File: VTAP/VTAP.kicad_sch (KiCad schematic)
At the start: 40 parts, among them J1 MX 52901-0274

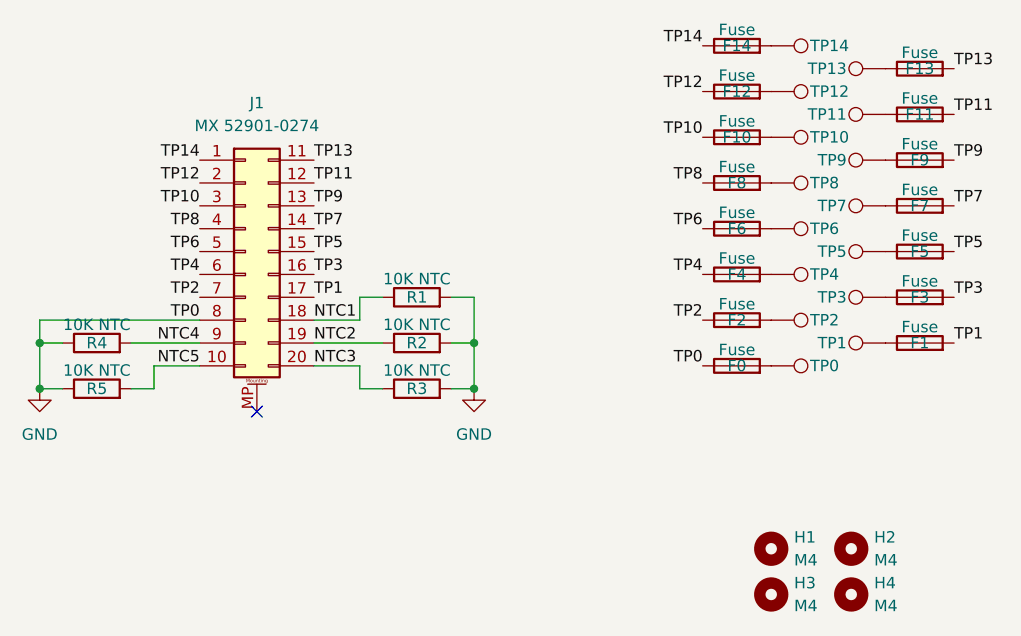
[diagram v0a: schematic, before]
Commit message: VTAP update
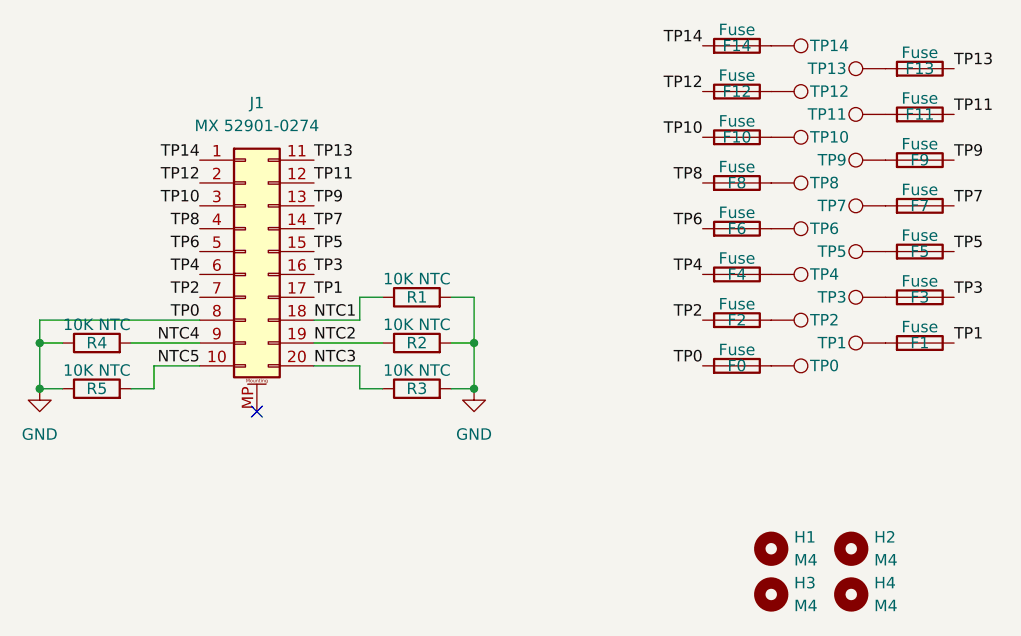
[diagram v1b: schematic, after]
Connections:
- net GND: now also F0.2; no longer F0.1
- net TP1: now also F1.1; no longer F1.2
- net TP10: now also F10.2; no longer F10.1
- net TP11: now also F11.1; no longer F11.2
- net TP12: now also F12.2; no longer F12.1
- net TP13: now also F13.1; no longer F13.2
- net TP14: now also F14.2; no longer F14.1
- net TP2: now also F2.2; no longer F2.1
- net TP3: now also F3.1; no longer F3.2
- net TP4: now also F4.2; no longer F4.1
- net TP5: now also F5.1; no longer F5.2
- net TP6: now also F6.2; no longer F6.1
- net TP7: now also F7.1; no longer F7.2
- net TP8: now also F8.2; no longer F8.1
- net TP9: now also F9.1; no longer F9.2
- net at TP12.1: now also F12.1; no longer F12.2
- net at TP1.1: now also F1.2; no longer F1.1
- net at TP13.1: now also F13.2; no longer F13.1
- net at TP11.1: now also F11.2; no longer F11.1
- net at TP6.1: now also F6.1; no longer F6.2
- net at TP5.1: now also F5.2; no longer F5.1
- net at TP7.1: now also F7.2; no longer F7.1
- net at TP4.1: now also F4.1; no longer F4.2
- net at TP8.1: now also F8.1; no longer F8.2
- net at TP14.1: now also F14.1; no longer F14.2
- net at TP10.1: now also F10.1; no longer F10.2
- net at TP2.1: now also F2.1; no longer F2.2
- net at TP3.1: now also F3.2; no longer F3.1
- net at TP0.1: now also F0.1; no longer F0.2
- net at TP9.1: now also F9.2; no longer F9.1
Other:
- moved on the sheet: F0, F1, F10, F11, F12, F13, F14, F2, F3, F4, F5, F6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
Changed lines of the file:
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@@
 	(symbol
 		(lib_id "Device:Fuse")
-		(at 219.71 111.76 90)
+		(at 219.71 111.76 270)
+		(mirror x)
 		(unit 1)
 		(exclude_from_sim no)
@@
 	(symbol
 		(lib_id "Device:Fuse")
-		(at 219.71 81.28 90)
+		(at 219.71 81.28 270)
+		(mirror x)
 		(unit 1)
 		(exclude_from_sim no)
@@
 	(symbol
 		(lib_id "Device:Fuse")
-		(at 219.71 86.36 90)
+		(at 219.71 86.36 270)
+		(mirror x)
 		(unit 1)
 		(exclude_from_sim no)
@@
 	(symbol
 		(lib_id "Device:Fuse")
-		(at 199.39 83.82 90)
+		(at 199.39 83.82 270)
+		(mirror x)
 		(unit 1)
 		(exclude_from_sim no)
@@
 	(symbol
 		(lib_id "Device:Fuse")
-		(at 219.71 96.52 90)
+		(at 219.71 96.52 270)
+		(mirror x)
 		(unit 1)
 		(exclude_from_sim no)
@@
 	(symbol
 		(lib_id "Device:Fuse")
-		(at 199.39 93.98 90)
+		(at 199.39 93.98 270)
+		(mirror x)
 		(unit 1)
 		(exclude_from_sim no)
@@
 	(symbol
 		(lib_id "Device:Fuse")
-		(at 199.39 104.14 90)
+		(at 199.39 104.14 270)
+		(mirror x)
 		(unit 1)
 		(exclude_from_sim no)
@@
 	(symbol
 		(lib_id "Device:Fuse")
-		(at 199.39 88.9 90)
+		(at 199.39 88.9 270)
+		(mirror x)
 		(unit 1)
 		(exclude_from_sim no)
@@
 	(symbol
 		(lib_id "Device:Fuse")
-		(at 199.39 109.22 90)
+		(at 199.39 109.22 270)
+		(mirror x)
 		(unit 1)
 		(exclude_from_sim no)
@@
 	(symbol
 		(lib_id "Device:Fuse")
-		(at 219.71 106.68 90)
+		(at 219.71 106.68 270)
+		(mirror x)
 		(unit 1)
 		(exclude_from_sim no)
@@
 	(symbol
 		(lib_id "Device:Fuse")
-		(at 219.71 91.44 90)
+		(at 219.71 91.44 270)
+		(mirror x)
 		(unit 1)
 		(exclude_from_sim no)
@@
 	(symbol
 		(lib_id "Device:Fuse")
-		(at 219.71 101.6 90)
+		(at 219.71 101.6 270)
+		(mirror x)
 		(unit 1)
 		(exclude_from_sim no)
@@
 	(symbol
 		(lib_id "Device:Fuse")
-		(at 199.39 114.3 90)
+		(at 199.39 114.3 270)
+		(mirror x)
 		(unit 1)
 		(exclude_from_sim no)
@@
 	(symbol
 		(lib_id "Device:Fuse")
-		(at 199.39 99.06 90)
+		(at 199.39 99.06 270)
+		(mirror x)
 		(unit 1)
 		(exclude_from_sim no)
@@
 	(symbol
 		(lib_id "Device:Fuse")
-		(at 199.39 78.74 90)
-		(unit 1)
-		(exclude_from_sim no)
+		(at 199.39 78.74 270)
+		(mirror x)
+		(unit 1)
+		(exclude_from_sim no)
